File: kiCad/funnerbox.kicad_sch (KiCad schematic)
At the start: 13 parts, among them J6 MIDI IN JACK, J7 EXPRESSION JACK, SW1 SW_SPDT, SW2 SW_SPDT, SW3 SW_SPDT

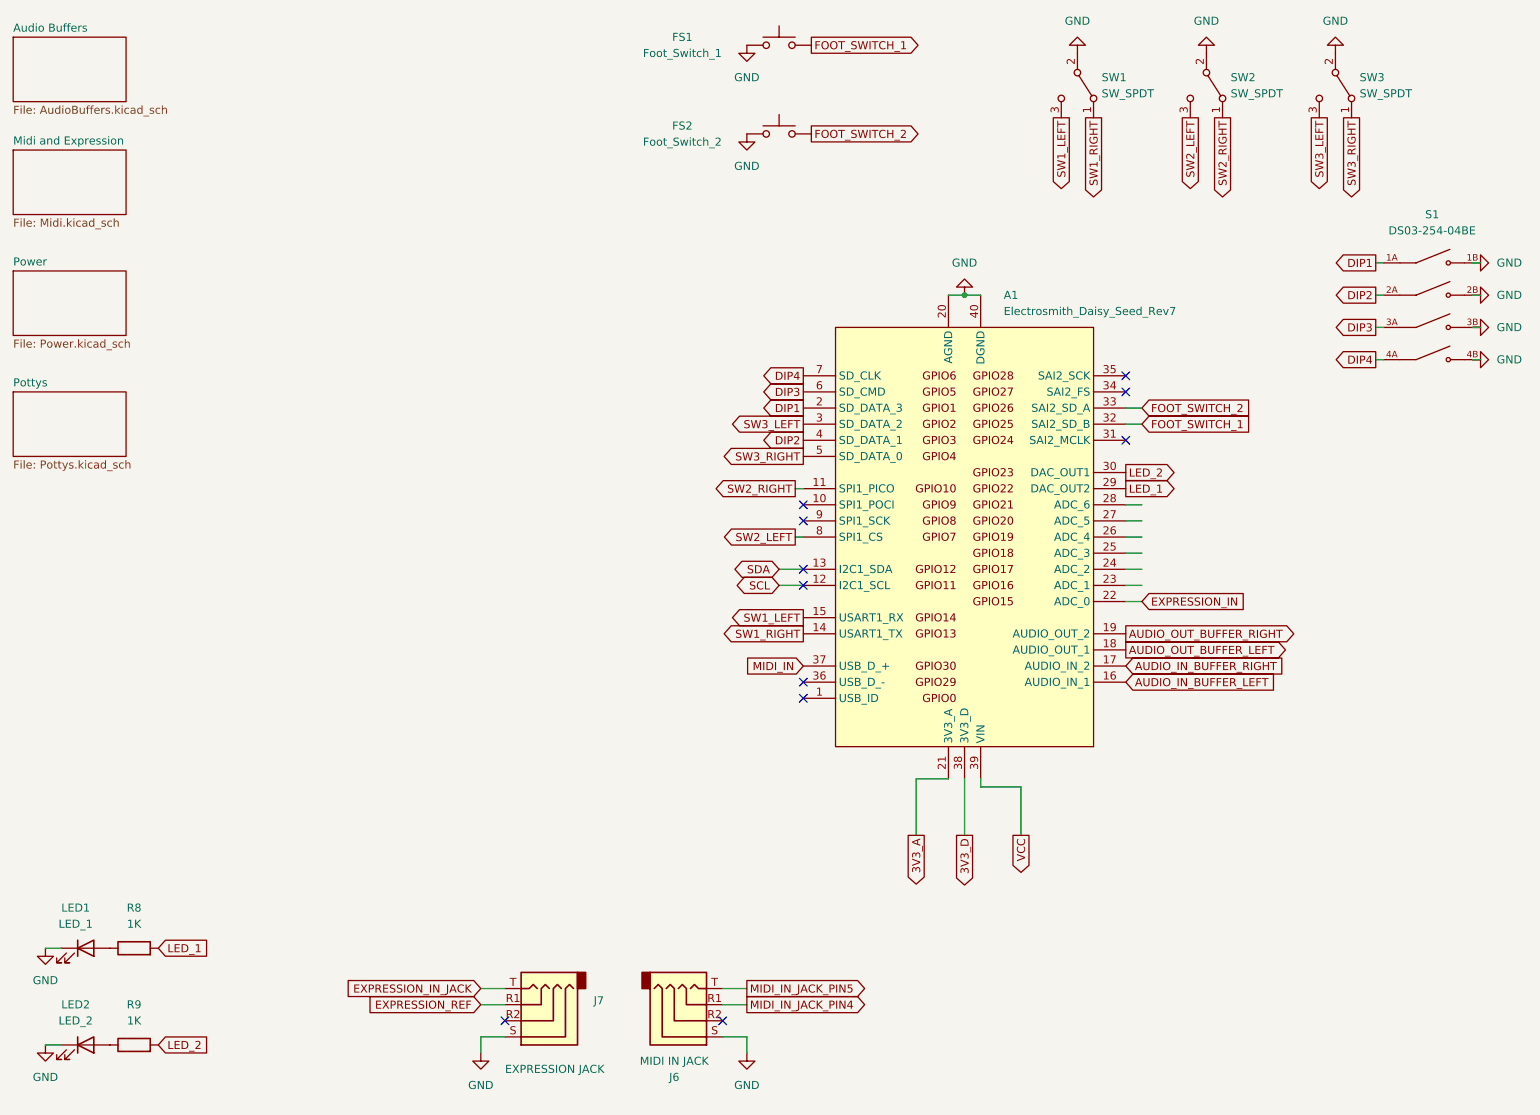
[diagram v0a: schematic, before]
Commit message: Updated kiCad Project
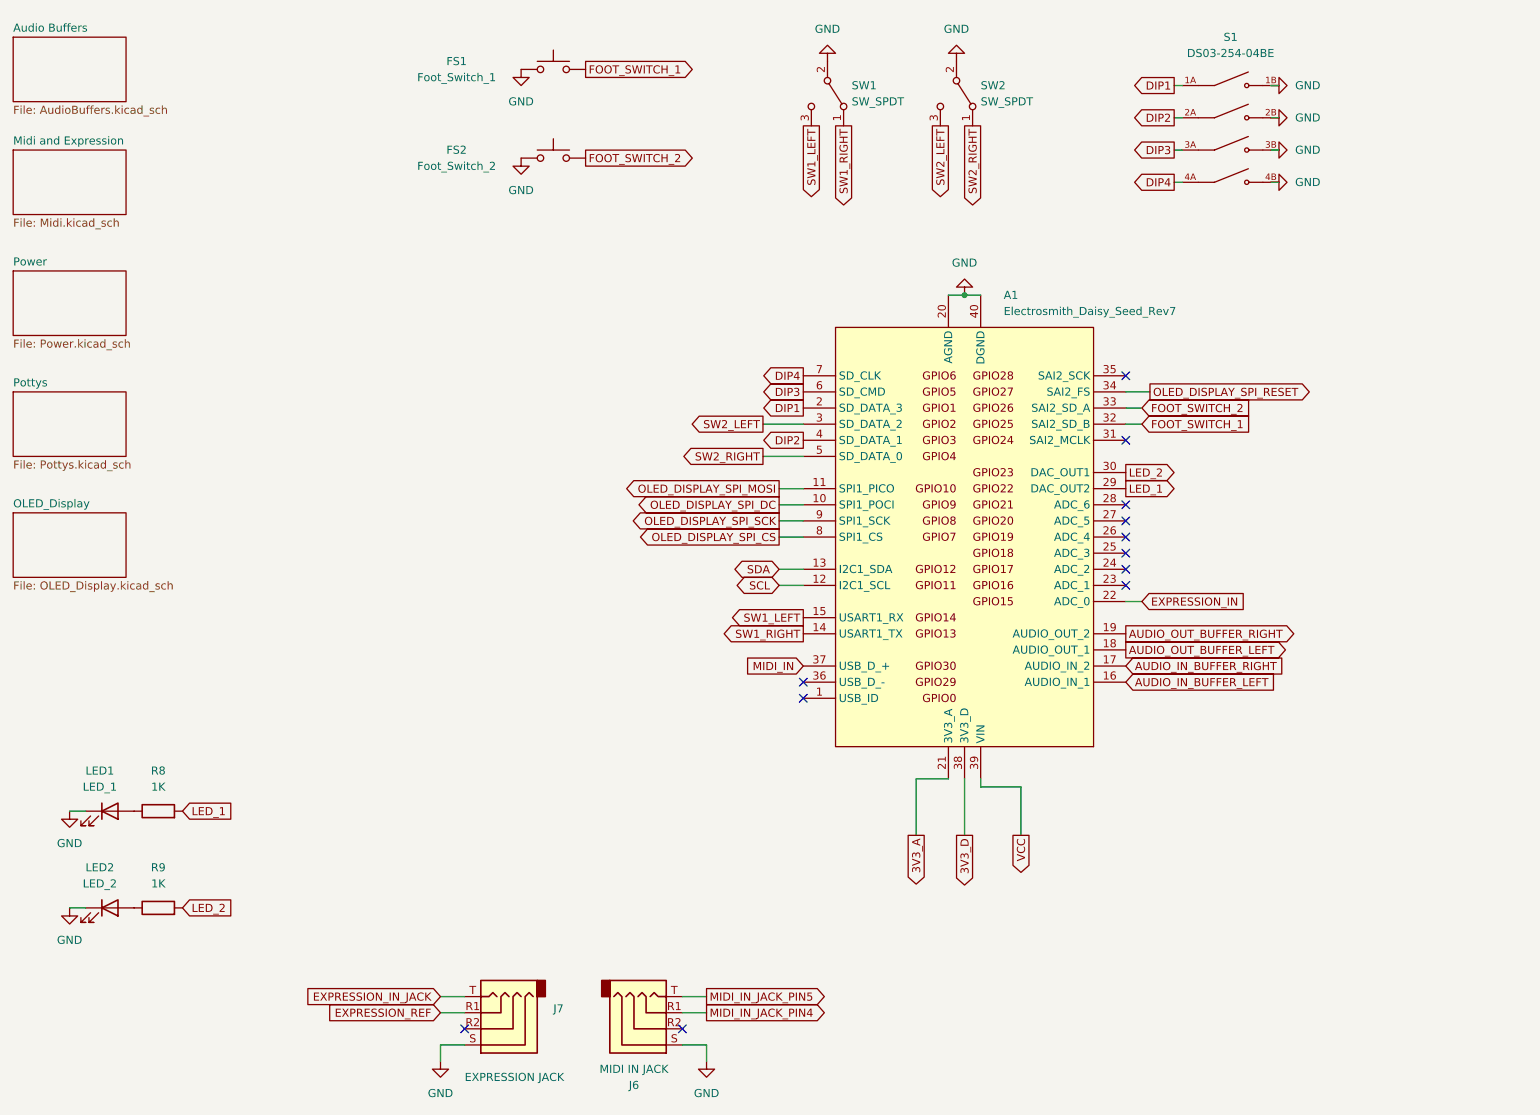
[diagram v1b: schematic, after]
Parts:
- removed SW3: SW_SPDT, Button_Switch_THT:SW_Toggle_SPDT_lugs, symbol Switch:SW_SPDT
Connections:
- net SW3_LEFT is gone; now on net SW2_LEFT: A1.3 (SD_DATA_2)
- net SW3_RIGHT is gone; now on net SW2_RIGHT: A1.5 (SD_DATA_0)
- net SW2_LEFT: no longer A1.8 (SPI1_CS)
- net SW2_RIGHT: no longer A1.11 (SPI1_PICO)
- net OLED_DISPLAY_SPI_DC: now reaches A1.10 (SPI1_POCI)
- net OLED_DISPLAY_SPI_RESET: now reaches A1.34 (SAI2_FS)
- net OLED_DISPLAY_SPI_SCK: now reaches A1.9 (SPI1_SCK)
- new net OLED_DISPLAY_SPI_CS: A1.8 (SPI1_CS)
- new net OLED_DISPLAY_SPI_MOSI: A1.11 (SPI1_PICO)
- no-connect marks 11 -> 12
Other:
- added sheet OLED_Display (OLED_Display.kicad_sch)
- moved on the sheet: FS1, FS2, J6, J7, LED1, LED2, R8, R9, S1, SW1, SW2

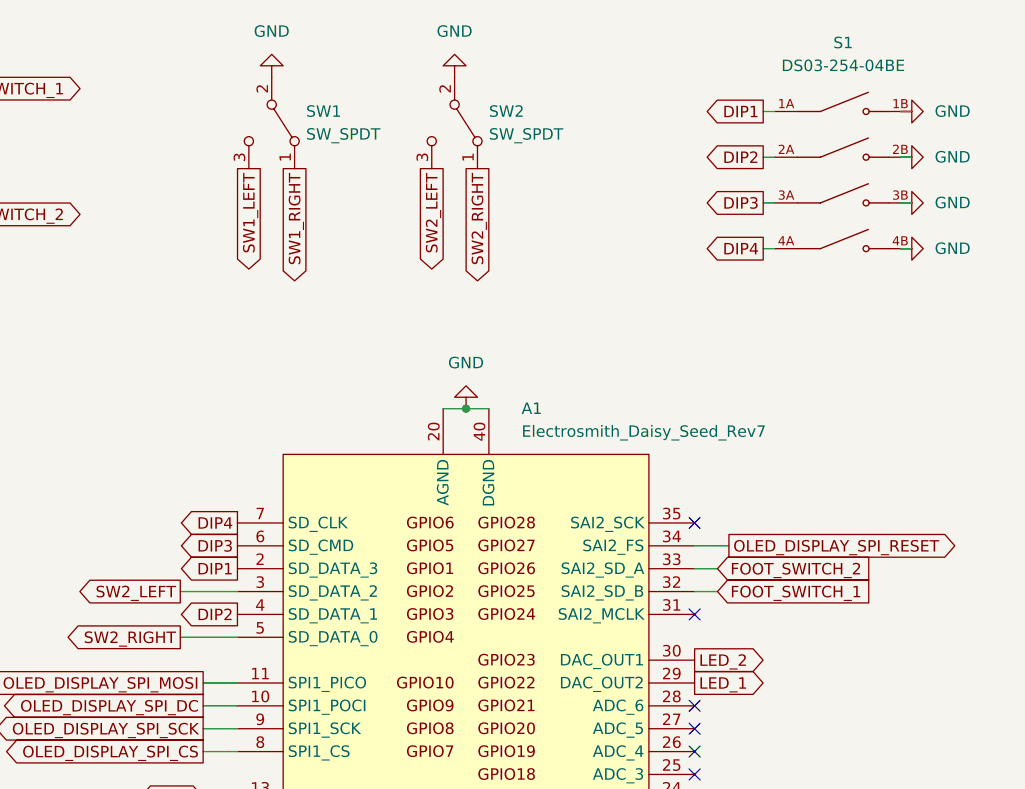
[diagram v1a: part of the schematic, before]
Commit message: Lots of stuff
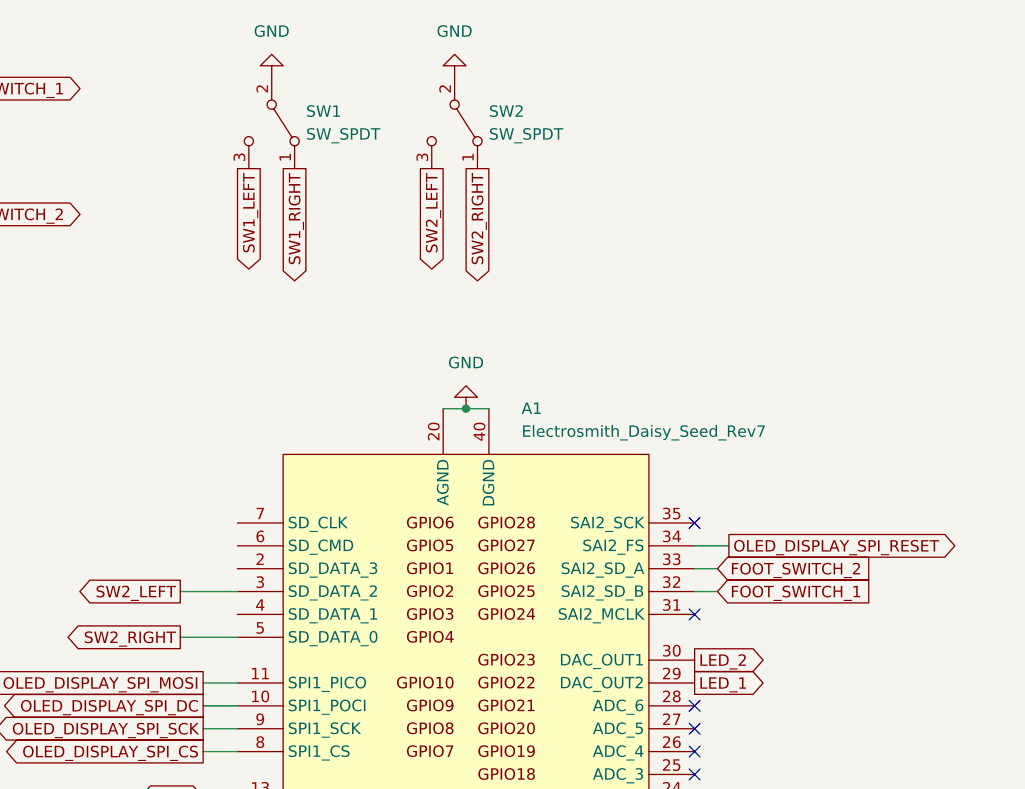
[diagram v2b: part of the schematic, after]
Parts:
- removed S1: DS03-254-04BE, Button_Switch_THT:DS03-254-04BE-dip4, symbol DS03-254-04BE:DS03-254-04BE
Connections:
- net DIP1: no longer names the net of A1.2 (SD_DATA_3)
- net DIP2: no longer names the net of A1.4 (SD_DATA_1)
- net DIP3: no longer names the net of A1.6 (SD_CMD)
- net DIP4: no longer names the net of A1.7 (SD_CLK)
